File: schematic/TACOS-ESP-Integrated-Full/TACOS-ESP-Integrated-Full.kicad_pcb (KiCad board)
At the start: 2 copper layers, 69.6 x 57.9 mm, 36 parts, among them J1 Power Relay, J2 MRC522, J4 Vin, Q1 PN2222A, Q2 PN2222A, Q3 PN2222A, Q4 PN2222A, Q5 PN2222A, SW1 SW_ARM, SW2 SW_DEVICE_RST, U1 WeMos_D1_mini

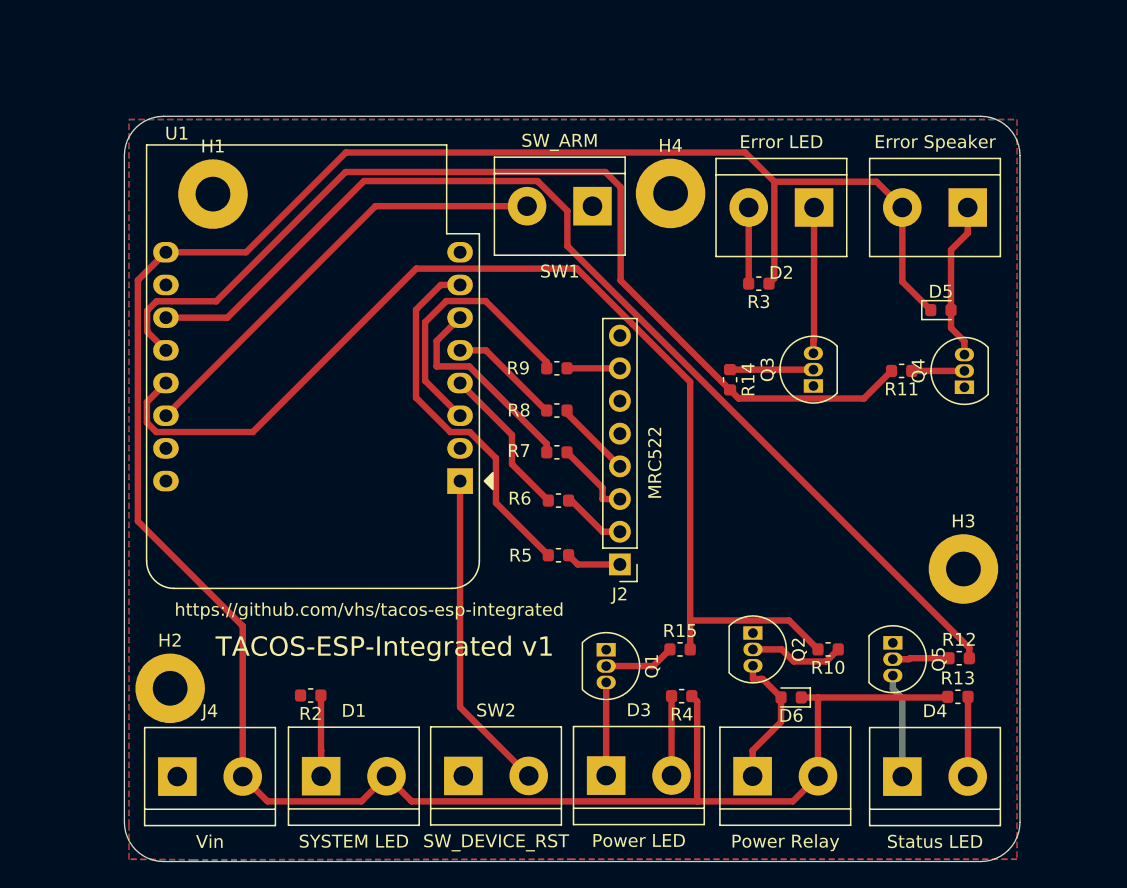
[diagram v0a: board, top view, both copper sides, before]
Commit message: schematic: updates
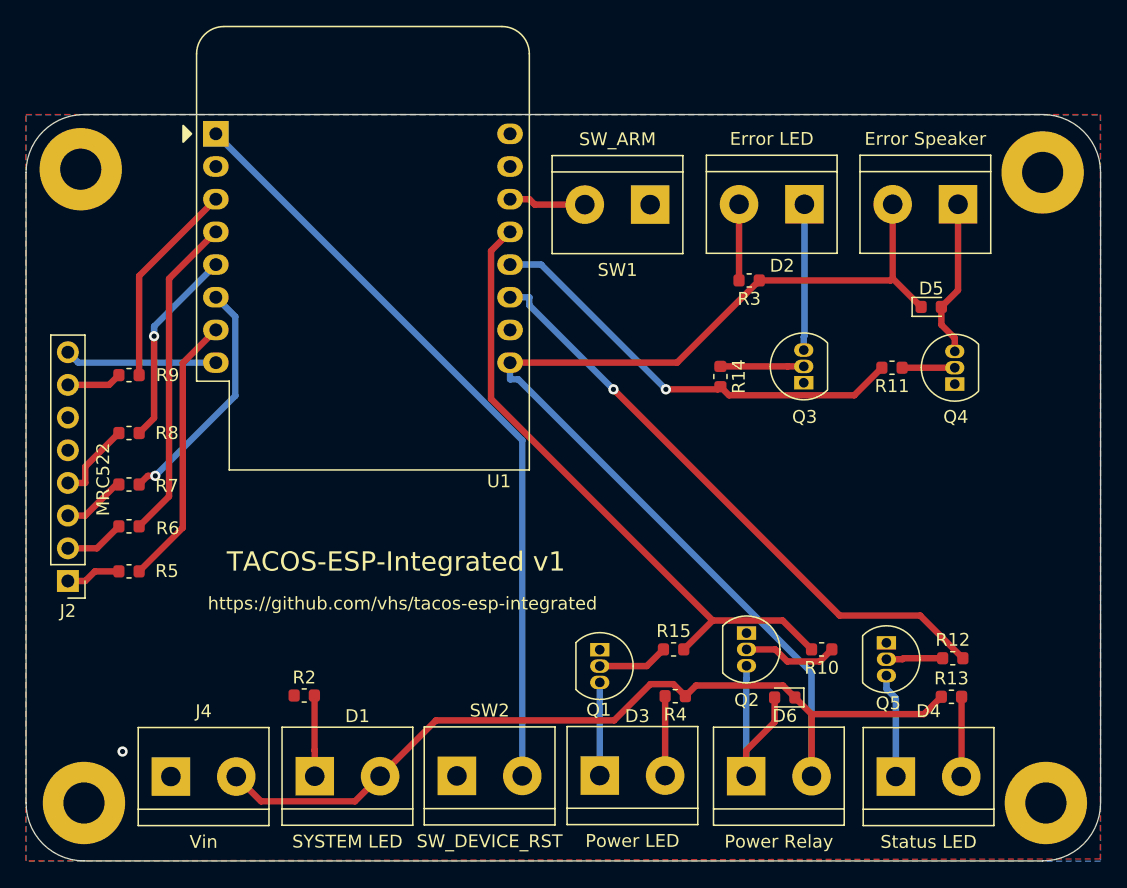
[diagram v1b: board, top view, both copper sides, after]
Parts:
- H1, H2, H3, H4: footprint MountingHole:MountingHole_2.7mm_M2.5_Pad -> MountingHole:MountingHole_3.2mm_M3_Pad
- moved J2 42.9 mm to (20.5, 60.8)
- moved R6 33.4 mm to (25.2, 56.5), turned to 180 degrees
- moved R5 33.4 mm to (25.2, 60.0), turned to 180 degrees
- moved R7 33.3 mm to (25.2, 53.2), turned to 180 degrees
- moved R8 33.3 mm to (25.2, 49.2), turned to 180 degrees
- moved R9 33.3 mm to (25.2, 44.8), turned to 180 degrees
- moved U1 33.0 mm to (32.0, 26.0), turned to 0 degrees
- moved H4 29.0 mm to (96.2, 29.0)
- moved H3 19.3 mm to (96.5, 78.0)
- moved H2 11.1 mm to (21.8, 78.0)
- moved H1 10.5 mm to (21.5, 28.8)
- moved SW1 4.49 mm to (65.8, 31.5)
- moved D2 0.79 mm to (77.7, 31.5)
- moved D5 0.79 mm to (87.6, 39.5)
- moved LS1 0.79 mm to (89.7, 31.5)
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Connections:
- J2 pad 8: (no net) -> +3V3
- U1 pad 8: (no net) -> +3V3
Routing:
- net +5V: track 198.0 -> 150.0 mm
- net ERROR_NET: track 78.4 -> 34.2 mm, vias 0 -> 1
- net STATUS_NET: track 84.3 -> 47.2 mm, vias 0 -> 1
- net POWER_NET: track 86.8 -> 49.7 mm
- net DEV_RST: track 25.1 -> 59.8 mm
- net SWITCH: track 34.8 -> 5.98 mm
- net SCK: track 12.0 -> 25.3 mm
- net +3V3: track 0.00 -> 11.8 mm
- net SS: track 28.4 -> 21.2 mm
- net MISO: track 8.67 -> 15.6 mm, vias 0 -> 1
- net RST: track 21.0 -> 16.1 mm
- net Net-(D6-Pad2): track 10.8 -> 15.6 mm
- net MOSI: track 16.3 -> 18.6 mm, vias 0 -> 1
- net Net-(J2-Pad3): track 6.13 -> 4.96 mm
- net GND: vias 0 -> 1
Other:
- board size 69.6 x 57.9 mm -> 83.5 x 58 mm
